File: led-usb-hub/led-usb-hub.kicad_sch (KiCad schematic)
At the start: 142 parts, among them J1 USBC_USB2.0, J2 RGBUSB_54-00266, J3 RGBUSB_54-00266, J4 RGBUSB_54-00266, J5 SWD, SW1 RESET, SW2 BOOLSEL, SW3 LED_EN, U1 RP2040, U10 TPD2EUSB30, U11 TPD2EUSB30, U12 TC54VN3002, U13 W25Q16JVSN, U2 TPS2042D, U3 TPS2042D, U4 TPS563257DRLR, U5 TPS563257DRLR, U6 TUSB2046IBVF, U7 TPD2EUSB30, U8 TPD2EUSB30, U9 TPD2EUSB30, Y1 12Mhz, Y2 6Mhz

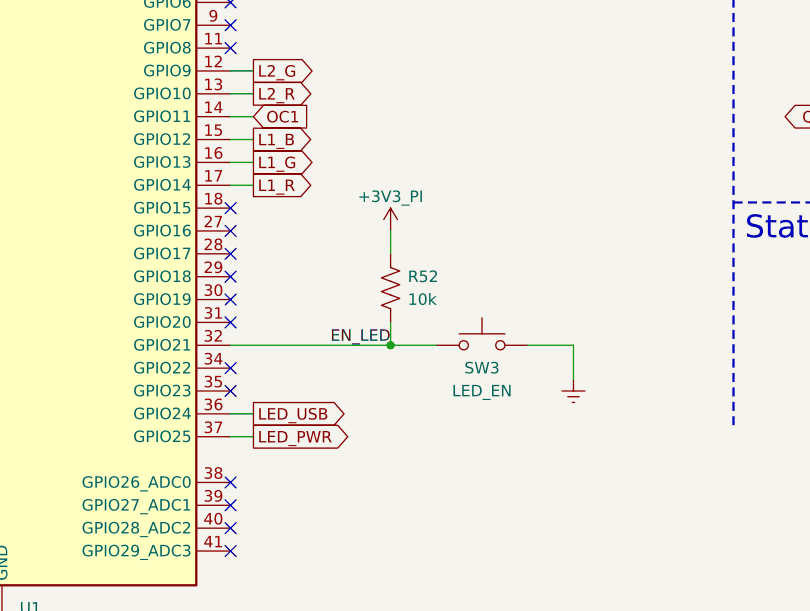
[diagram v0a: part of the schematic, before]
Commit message: Even more goddamn clean up and closer placement of decoupling caps
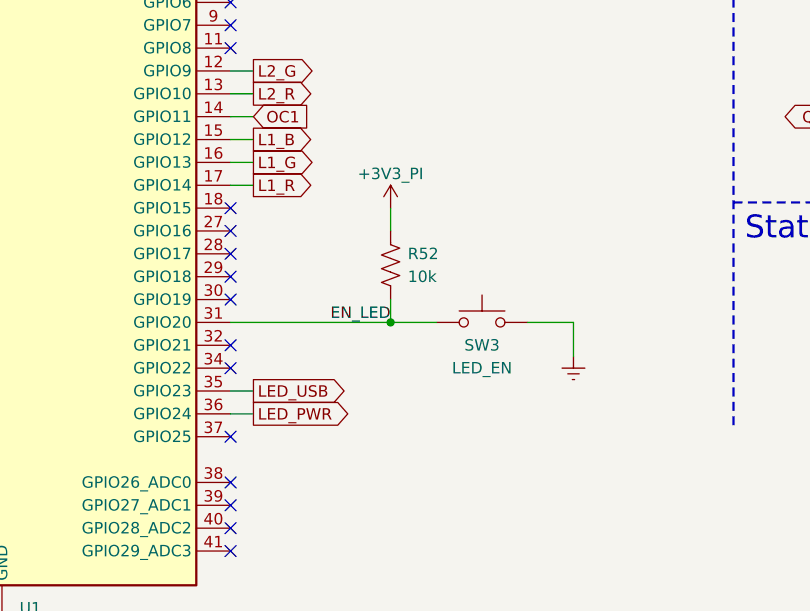
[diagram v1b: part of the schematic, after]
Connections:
- net EN_LED: now also U1.31 (GPIO20); no longer U1.32 (GPIO21)
- net LED_PWR: now also U1.36 (GPIO24); no longer U1.37 (GPIO25)
- net LED_USB: now also U1.35 (GPIO23); no longer U1.36 (GPIO24)
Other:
- moved on the sheet: R52, SW3
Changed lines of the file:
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@@
   (junction (at 33.02 82.55) (diameter 0) (color 0 0 0 0)
   )
-  (junction (at 299.72 243.84) (diameter 0) (color 0 0 0 0)
+  (junction (at 299.72 241.3) (diameter 0) (color 0 0 0 0)
   )
   (junction (at 158.75 146.05) (diameter 0) (color 0 0 0 0)
@@
   (no_connect (at 281.94 210.82))
   (no_connect (at 281.94 236.22))
-  (no_connect (at 281.94 248.92))
+  (no_connect (at 281.94 254))
   (no_connect (at 247.65 90.17))
   (no_connect (at 281.94 208.28))
-  (no_connect (at 281.94 241.3))
+  (no_connect (at 281.94 243.84))
   (bus_entry (at 360.68 199.39) (size -2.54 2.54)
     (stroke (width 0) (type default))
@@
     (stroke (width 0) (type default))
   )
-  (wire (pts (xy 299.72 243.84) (xy 304.8 243.84))
+  (wire (pts (xy 299.72 241.3) (xy 304.8 241.3))
     (stroke (width 0) (type default))
   )
@@
     (stroke (width 0) (type default))
   )
-  (wire (pts (xy 281.94 243.84) (xy 299.72 243.84))
+  (wire (pts (xy 281.94 241.3) (xy 299.72 241.3))
     (stroke (width 0) (type default))
   )
@@
     (stroke (width 0) (type default))
   )
-  (wire (pts (xy 284.48 254) (xy 281.94 254))
+  (wire (pts (xy 284.48 251.46) (xy 281.94 251.46))
     (stroke (width 0) (type default))
   )
@@
     (stroke (width 0) (type default))
   )
-  (wire (pts (xy 299.72 241.3) (xy 299.72 243.84))
+  (wire (pts (xy 299.72 238.76) (xy 299.72 241.3))
     (stroke (width 0) (type default))
   )
@@
     (stroke (width 0) (type default))
   )
-  (wire (pts (xy 299.72 233.68) (xy 299.72 231.14))
+  (wire (pts (xy 299.72 231.14) (xy 299.72 228.6))
     (stroke (width 0) (type default))
   )
@@
     (stroke (width 0) (type default))
   )
-  (wire (pts (xy 284.48 251.46) (xy 281.94 251.46))
+  (wire (pts (xy 284.48 248.92) (xy 281.94 248.92))
     (stroke (width 0) (type default))
   )
@@
     (stroke (width 0) (type default))
   )
-  (wire (pts (xy 314.96 243.84) (xy 320.04 243.84))
+  (wire (pts (xy 314.96 241.3) (xy 320.04 241.3))
     (stroke (width 0) (type default))
   )
@@
     (stroke (width 0) (type default))
   )
-  (wire (pts (xy 320.04 243.84) (xy 320.04 247.65))
+  (wire (pts (xy 320.04 241.3) (xy 320.04 245.11))
     (stroke (width 0) (type default))
   )
@@
     (effects (font (size 1.27 1.27) (color 0 0 194 0)) (justify right bottom))
   )
-  (label "EN_LED" (at 299.72 243.84 180) (fields_autoplaced)
+  (label "EN_LED" (at 299.72 241.3 180) (fields_autoplaced)
     (effects (font (size 1.27 1.27) (color 0 0 194 0)) (justify right bottom))
   )
@@
     )
   )
-  (global_label "LED_USB" (shape output) (at 284.48 251.46 0) (fields_autoplaced)
+  (global_label "LED_USB" (shape output) (at 284.48 248.92 0) (fields_autoplaced)
     (effects (font (size 1.27 1.27)) (justify left))
-    (property "Intersheetrefs" "${INTERSHEET_REFS}" (at 295.6105 251.46 0)
+    (property "Intersheetrefs" "${INTERSHEET_REFS}" (at 295.6105 248.92 0)
       (effects (font (size 1.27 1.27)) (justify left) hide)
     )
@@
     )
   )
-  (global_label "LED_PWR" (shape output) (at 284.48 254 0) (fields_autoplaced)
+  (global_label "LED_PWR" (shape output) (at 284.48 251.46 0) (fields_autoplaced)
     (effects (font (size 1.27 1.27)) (justify left))
-    (property "Intersheetrefs" "${INTERSHEET_REFS}" (at 295.7919 254 0)
+    (property "Intersheetrefs" "${INTERSHEET_REFS}" (at 295.7919 251.46 0)
       (effects (font (size 1.27 1.27)) (justify left) hide)
     )
@@
     )
   )
-  (symbol (lib_id "Switch:SW_Push") (at 309.88 243.84 0) (unit 1)
+  (symbol (lib_id "Switch:SW_Push") (at 309.88 241.3 0) (unit 1)
     (in_bom yes) (on_board yes) (dnp no)
-    (property "Reference" "SW3" (at 309.88 246.38 0)
+    (property "Reference" "SW3" (at 309.88 243.84 0)
       (effects (font (size 1.27 1.27)))
     )
-    (property "Value" "LED_EN" (at 309.88 248.92 0)
+    (property "Value" "LED_EN" (at 309.88 246.38 0)
       (effects (font (size 1.27 1.27)))
     )
-    (property "Footprint" "KSS221GLFS:SW_KSS221GLFS" (at 309.88 238.76 0)
+    (property "Footprint" "KSS221GLFS:SW_KSS221GLFS" (at 309.88 236.22 0)
       (effects (font (size 1.27 1.27)) hide)
     )
-    (property "Datasheet" "~" (at 309.88 238.76 0)
+    (property "Datasheet" "~" (at 309.88 236.22 0)
       (effects (font (size 1.27 1.27)) hide)
     )
@@
     )
   )
-  (symbol (lib_id "power:Earth") (at 320.04 247.65 0) (unit 1)
+  (symbol (lib_id "power:Earth") (at 320.04 245.11 0) (unit 1)
     (in_bom yes) (on_board yes) (dnp no) (fields_autoplaced)
-    (property "Reference" "#PWR045" (at 320.04 254 0)
+    (property "Reference" "#PWR045" (at 320.04 251.46 0)
       (effects (font (size 1.27 1.27)) hide)
     )
-    (property "Value" "Earth" (at 320.04 251.46 0)
+    (property "Value" "Earth" (at 320.04 248.92 0)
       (effects (font (size 1.27 1.27)) hide)
     )
-    (property "Footprint" "" (at 320.04 247.65 0)
+    (property "Footprint" "" (at 320.04 245.11 0)
       (effects (font (size 1.27 1.27)) hide)
     )
-    (property "Datasheet" "~" (at 320.04 247.65 0)
+    (property "Datasheet" "~" (at 320.04 245.11 0)
       (effects (font (size 1.27 1.27)) hide)
     )
@@
     )
   )
-  (symbol (lib_id "power:+3V3_PI") (at 299.72 231.14 0) (unit 1)
+  (symbol (lib_id "power:+3V3_PI") (at 299.72 228.6 0) (unit 1)
     (in_bom yes) (on_board yes) (dnp no) (fields_autoplaced)
-    (property "Reference" "#PWR065" (at 299.72 234.95 0)
+    (property "Reference" "#PWR065" (at 299.72 232.41 0)
       (effects (font (size 1.27 1.27)) hide)
     )
-    (property "Value" "+3V3_PI" (at 299.72 227.33 0)
+    (property "Value" "+3V3_PI" (at 299.72 224.79 0)
       (effects (font (size 1.27 1.27)))
     )
-    (property "Footprint" "" (at 299.72 231.14 0)
+    (property "Footprint" "" (at 299.72 228.6 0)
       (effects (font (size 1.27 1.27)) hide)
     )
-    (property "Datasheet" "" (at 299.72 231.14 0)
+    (property "Datasheet" "" (at 299.72 228.6 0)
       (effects (font (size 1.27 1.27)) hide)
     )
@@
     )
   )
-  (symbol (lib_id "Device:R_US") (at 299.72 237.49 0) (unit 1)
+  (symbol (lib_id "Device:R_US") (at 299.72 234.95 0) (unit 1)
     (in_bom yes) (on_board yes) (dnp no)
-    (property "Reference" "R52" (at 301.625 236.22 0)
+    (property "Reference" "R52" (at 301.625 233.68 0)
       (effects (font (size 1.27 1.27)) (justify left))
     )
-    (property "Value" "10k" (at 301.625 238.76 0)
+    (property "Value" "10k" (at 301.625 236.22 0)
       (effects (font (size 1.27 1.27)) (justify left))
     )
-    (property "Footprint" "Resistor_SMD:R_0603_1608Metric" (at 300.736 237.744 90)
+    (property "Footprint" "Resistor_SMD:R_0603_1608Metric" (at 300.736 235.204 90)
       (effects (font (size 1.27 1.27)) hide)
     )
-    (property "Datasheet" "~" (at 299.72 237.49 0)
+    (property "Datasheet" "~" (at 299.72 234.95 0)
       (effects (font (size 1.27 1.27)) hide)
     )

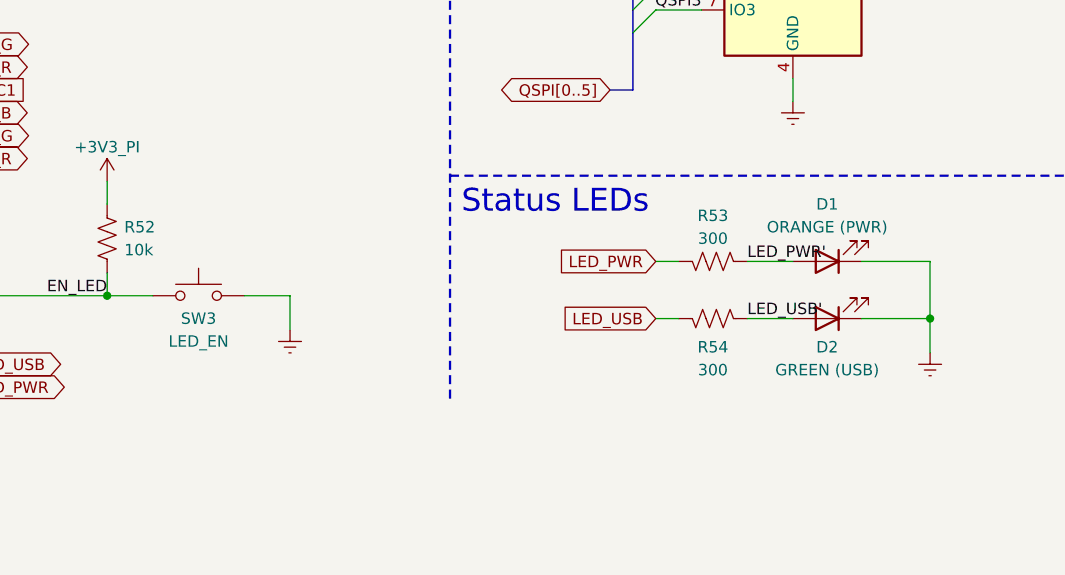
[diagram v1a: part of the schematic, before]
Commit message: Clean up and aligning
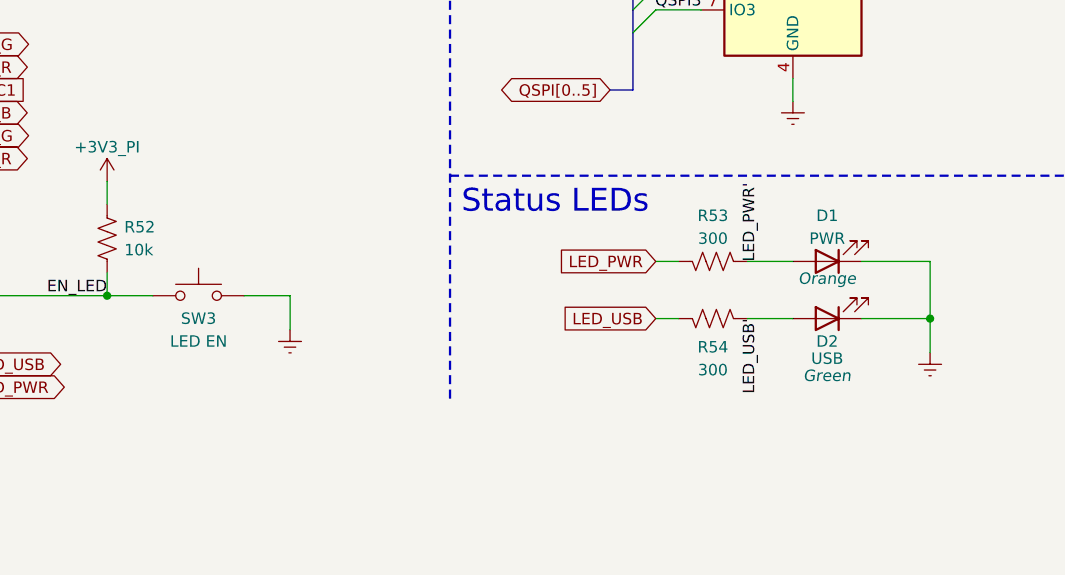
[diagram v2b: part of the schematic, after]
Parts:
- D1: value ORANGE (PWR) -> PWR; Color (none) -> Orange
- D2: value GREEN (USB) -> USB; Color (none) -> Green
- SW3: value LED_EN -> LED EN
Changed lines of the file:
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@@
     (effects (font (size 1.27 1.27) (color 0 0 255 0)) (justify left bottom))
   )
-  (label "LED_USB'" (at 370.84 243.84 0) (fields_autoplaced)
-    (effects (font (size 1.27 1.27) (color 0 0 255 0)) (justify left bottom))
+  (label "LED_USB'" (at 372.11 243.84 270) (fields_autoplaced)
+    (effects (font (size 1.27 1.27) (color 0 0 255 0)) (justify right bottom))
   )
   (label "CC1" (at 46.99 31.75 0) (fields_autoplaced)
@@
     (effects (font (size 1.27 1.27) (color 0 0 255 0)) (justify left bottom))
   )
-  (label "LED_PWR'" (at 370.84 237.49 0) (fields_autoplaced)
+  (label "LED_PWR'" (at 372.11 237.49 90) (fields_autoplaced)
     (effects (font (size 1.27 1.27) (color 0 0 255 0)) (justify left bottom))
   )
@@
       (effects (font (size 1.27 1.27)))
     )
-    (property "Value" "LED_EN" (at 309.88 246.38 0)
+    (property "Value" "LED EN" (at 309.88 246.38 0)
       (effects (font (size 1.27 1.27)))
     )
@@
   (symbol (lib_id "Device:LED") (at 379.73 237.49 180) (unit 1)
     (in_bom yes) (on_board yes) (dnp no)
-    (property "Reference" "D1" (at 379.73 231.14 0)
+    (property "Reference" "D1" (at 379.73 232.41 0)
       (effects (font (size 1.27 1.27)))
     )
-    (property "Value" "ORANGE (PWR)" (at 379.73 233.68 0)
+    (property "Value" "PWR" (at 379.73 234.95 0)
       (effects (font (size 1.27 1.27)))
     )
@@
       (effects (font (size 1.27 1.27)) hide)
     )
+    (property "Color" "Orange" (at 379.73 239.395 0)
+      (effects (font (size 1.27 1.27) italic))
+    )
     (pin "1")
     (pin "2")
@@
   (symbol (lib_id "Device:LED") (at 379.73 243.84 180) (unit 1)
     (in_bom yes) (on_board yes) (dnp no)
-    (property "Reference" "D2" (at 379.73 247.015 0)
+    (property "Reference" "D2" (at 379.73 246.38 0)
       (effects (font (size 1.27 1.27)))
     )
-    (property "Value" "GREEN (USB)" (at 379.73 249.555 0)
+    (property "Value" "USB" (at 379.73 248.285 0)
       (effects (font (size 1.27 1.27)))
     )
@@
       (effects (font (size 1.27 1.27)) hide)
     )
+    (property "Color" "Green" (at 379.73 250.19 0)
+      (effects (font (size 1.27 1.27) italic))
+    )
     (pin "1")
